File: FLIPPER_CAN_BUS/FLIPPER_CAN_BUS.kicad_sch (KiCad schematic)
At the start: 21 parts, among them J1 Conn_01x02, J1 Conn_01x08_Socket, J2 Conn_01x10_Socket, U1 TJA1051T/3, U2 MCP2515-xST, U3 AP3602AKTR-G1, Y1 16 Mhz

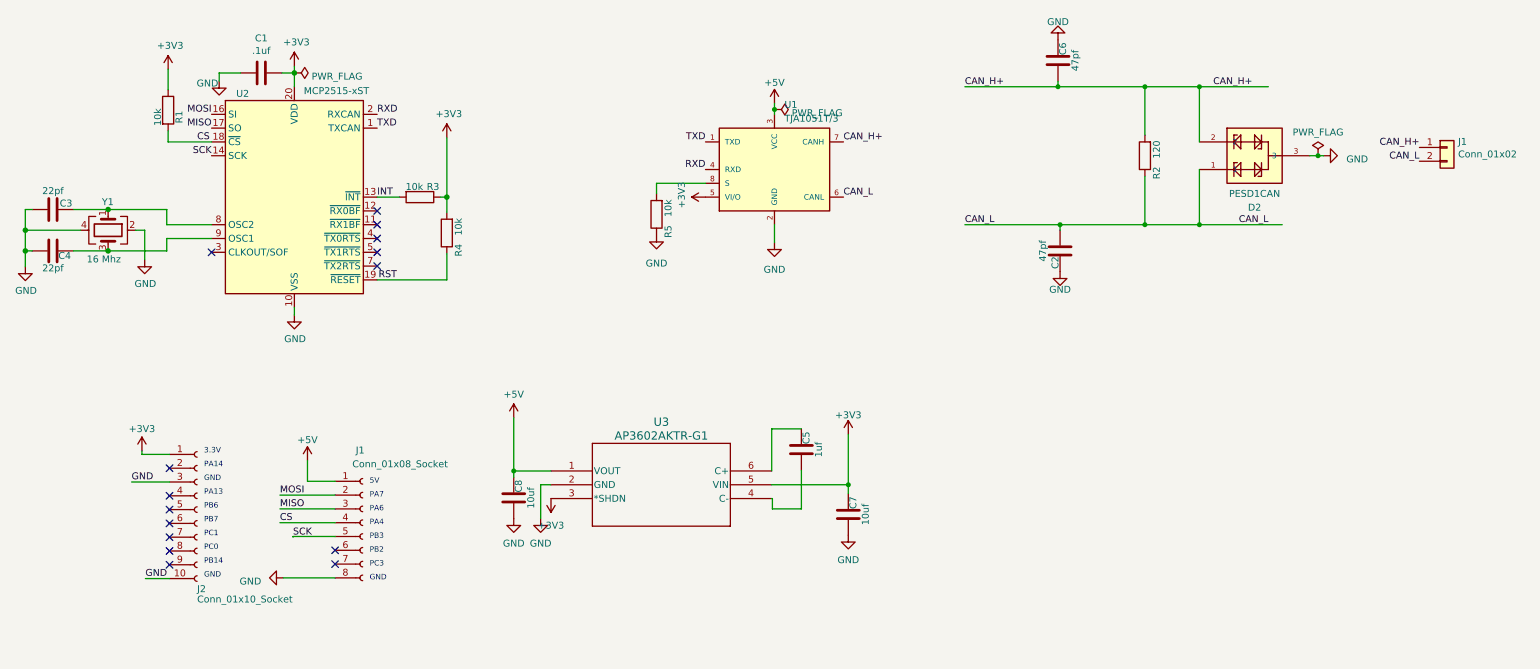
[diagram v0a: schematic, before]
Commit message: FLIPPER_CAN_BUS
Cambios en diseño
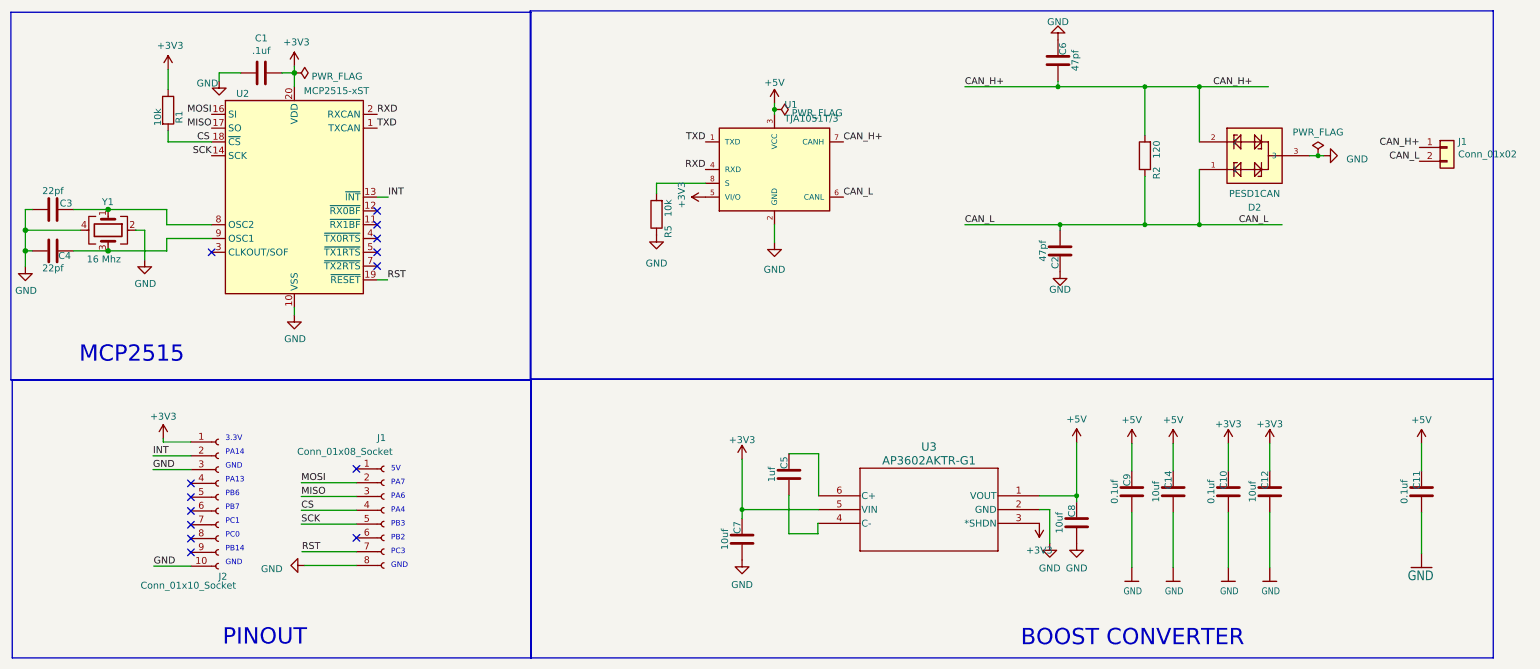
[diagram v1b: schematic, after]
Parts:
- removed R3, R4: 10k, Resistor_SMD:R_0603_1608Metric_Pad0.98x0.95mm_HandSolder, symbol CanBus-rescue:R-Device
- added C10, C11, C9: 0.1uf, Capacitor_SMD:C_0603_1608Metric_Pad1.08x0.95mm_HandSolder, symbol CanBus-rescue:C-Device
- added C12, C14: 10uf, Capacitor_SMD:C_0603_1608Metric_Pad1.08x0.95mm_HandSolder, symbol CanBus-rescue:C-Device
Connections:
- net +3V3: now also C10.1, C12.1
- net +5V: now also C11.1, C14.1, C9.1; no longer J1.1 (Pin_1)
- net GND: now also C10.2, C11.2, C12.2, C14.2, C9.2
- net INT: now also J2.2 (Pin_2)
- net RST: now also J1.7 (Pin_7)
- no-connect marks 15 -> 14
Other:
- note added: "BOOST CONVERTER"
- note added: "MCP2515"
- note added: "PINOUT"
- moved on the sheet: C5, C7, C8, J1, J2, U3
